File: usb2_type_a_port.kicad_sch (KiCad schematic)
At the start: 8 parts

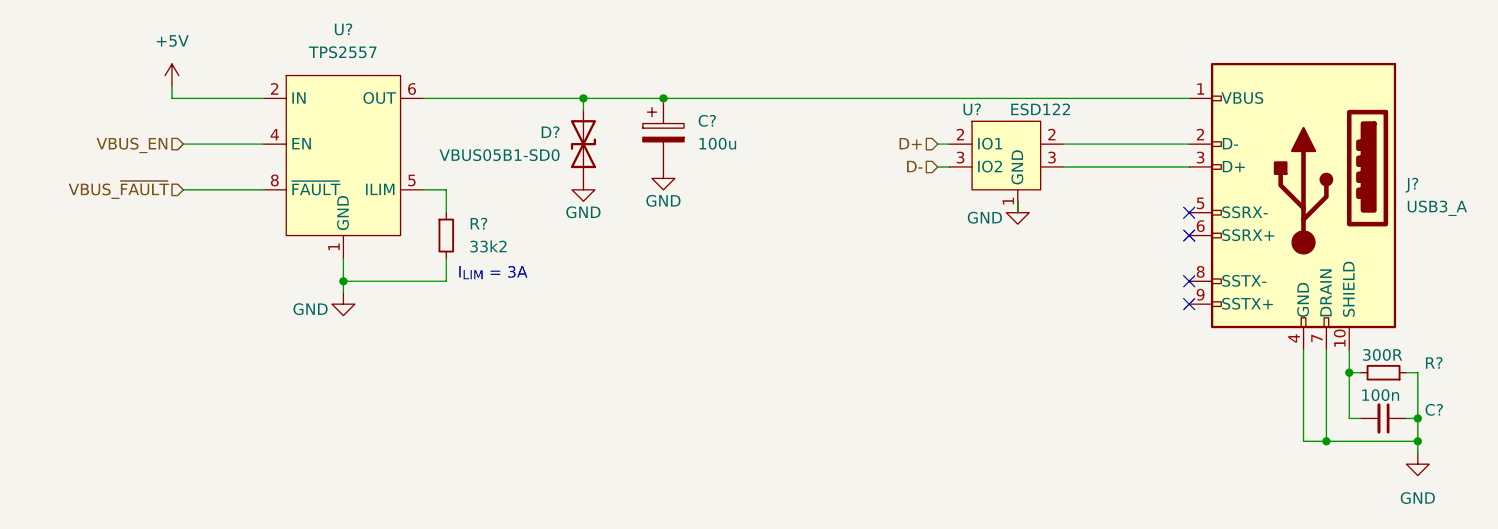
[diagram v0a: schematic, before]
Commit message: idk
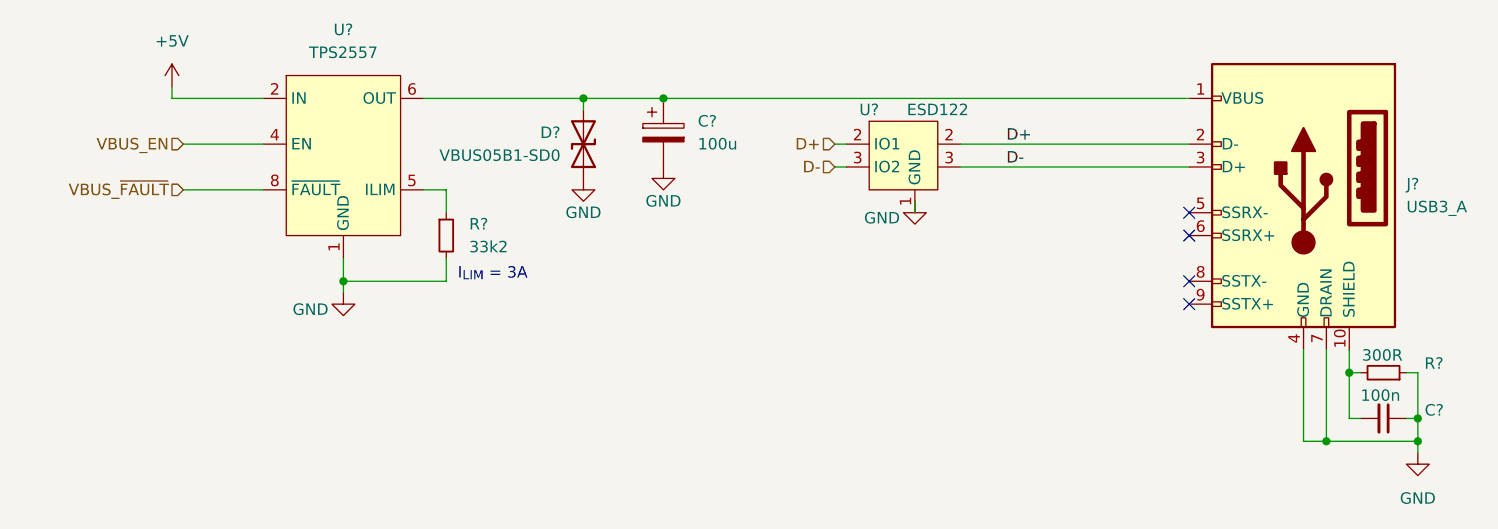
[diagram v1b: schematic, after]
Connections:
- net D+: now also J?.2 (D-)
- net D-: now also J?.3 (D+)
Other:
- moved on the sheet: U?
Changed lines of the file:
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@@
     (stroke (width 0) (type default))
   )
-  (wire (pts (xy 182.88 57.15) (xy 184.15 57.15))
-    (stroke (width 0) (type default))
-  )
-  (wire (pts (xy 196.85 54.61) (xy 210.82 54.61))
+  (wire (pts (xy 171.45 57.15) (xy 172.72 57.15))
+    (stroke (width 0) (type default))
+  )
+  (wire (pts (xy 185.42 54.61) (xy 210.82 54.61))
     (stroke (width 0) (type default))
   )
@@
     (stroke (width 0) (type default))
   )
-  (wire (pts (xy 182.88 54.61) (xy 184.15 54.61))
-    (stroke (width 0) (type default))
-  )
-  (wire (pts (xy 191.77 60.96) (xy 191.77 62.23))
-    (stroke (width 0) (type default))
-  )
-  (wire (pts (xy 196.85 57.15) (xy 210.82 57.15))
+  (wire (pts (xy 171.45 54.61) (xy 172.72 54.61))
+    (stroke (width 0) (type default))
+  )
+  (wire (pts (xy 180.34 60.96) (xy 180.34 62.23))
+    (stroke (width 0) (type default))
+  )
+  (wire (pts (xy 185.42 57.15) (xy 210.82 57.15))
     (stroke (width 0) (type default))
   )
@@
     (effects (font (size 1.27 1.27)) (justify left bottom))
   )
+  (label "D-" (at 190.5 57.15 0) (fields_autoplaced)
+    (effects (font (size 1.27 1.27)) (justify left bottom))
+  )
+  (label "D+" (at 190.5 54.61 0) (fields_autoplaced)
+    (effects (font (size 1.27 1.27)) (justify left bottom))
+  )
   (hierarchical_label "VBUS_EN" (shape input) (at 99.06 54.61 180) (fields_autoplaced)
     (effects (font (size 1.27 1.27)) (justify right))
   )
-  (hierarchical_label "D-" (shape input) (at 182.88 57.15 180) (fields_autoplaced)
+  (hierarchical_label "D-" (shape input) (at 171.45 57.15 180) (fields_autoplaced)
     (effects (font (size 1.27 1.27)) (justify right))
   )
-  (hierarchical_label "D+" (shape input) (at 182.88 54.61 180) (fields_autoplaced)
+  (hierarchical_label "D+" (shape input) (at 171.45 54.61 180) (fields_autoplaced)
     (effects (font (size 1.27 1.27)) (justify right))
   )
@@
     )
   )
-  (symbol (lib_id "Interface_USB:ESD122") (at 191.77 54.61 0) (unit 1)
+  (symbol (lib_id "Interface_USB:ESD122") (at 180.34 54.61 0) (unit 1)
     (in_bom yes) (on_board yes) (dnp no)
-    (property "Reference" "U?" (at 186.69 50.8 0)
-      (effects (font (size 1.27 1.27)))
-    )
-    (property "Value" "ESD122" (at 194.31 50.8 0)
-      (effects (font (size 1.27 1.27)))
-    )
-    (property "Footprint" "Package_SON:X2SON-3_L1.0-W0.6-L" (at 196.85 59.69 0)
-      (effects (font (size 1.27 1.27)) hide)
-    )
-    (property "Datasheet" "" (at 196.85 59.69 0)
-      (effects (font (size 1.27 1.27)) hide)
-    )
-    (property "LCSC" "C544474" (at 191.77 54.61 0)
-      (effects (font (size 1.27 1.27)) hide)
-    )
-    (property "MPN" "ESD122DMXR" (at 191.77 54.61 0)
+    (property "Reference" "U?" (at 175.26 50.8 0)
+      (effects (font (size 1.27 1.27)))
+    )
+    (property "Value" "ESD122" (at 182.88 50.8 0)
+      (effects (font (size 1.27 1.27)))
+    )
+    (property "Footprint" "Package_SON:X2SON-3_L1.0-W0.6-L" (at 185.42 59.69 0)
+      (effects (font (size 1.27 1.27)) hide)
+    )
+    (property "Datasheet" "" (at 185.42 59.69 0)
+      (effects (font (size 1.27 1.27)) hide)
+    )
+    (property "LCSC" "C544474" (at 180.34 54.61 0)
+      (effects (font (size 1.27 1.27)) hide)
+    )
+    (property "MPN" "ESD122DMXR" (at 180.34 54.61 0)
       (effects (font (size 1.27 1.27)) hide)
     )
@@
     )
   )
-  (symbol (lib_id "power:GND") (at 191.77 60.96 0) (unit 1)
+  (symbol (lib_id "power:GND") (at 180.34 60.96 0) (unit 1)
     (in_bom yes) (on_board yes) (dnp no)
-    (property "Reference" "#PWR?" (at 191.77 67.31 0)
-      (effects (font (size 1.27 1.27)) hide)
-    )
-    (property "Value" "GND" (at 188.1184 62.8331 0)
-      (effects (font (size 1.27 1.27)))
-    )
-    (property "Footprint" "" (at 191.77 60.96 0)
-      (effects (font (size 1.27 1.27)) hide)
-    )
-    (property "Datasheet" "" (at 191.77 60.96 0)
-      (effects (font (size 1.27 1.27)) hide)
-    )
+    (property "Reference" "#PWR?" (at 180.34 67.31 0)
+      (effects (font (size 1.27 1.27)) hide)
+    )
+    (property "Value" "GND" (at 176.6884 62.8331 0)
+      (effects (font (size 1.27 1.27)))
+    )
+    (property "Footprint" "" (at 180.34 60.96 0)
+      (effects (font (size 1.27 1.27)) hide)
+    )
+    (property "Datasheet" "" (at 180.34 60.96 0)
+      (effects (font (size 1.27 1.27)) hide)
+    )
